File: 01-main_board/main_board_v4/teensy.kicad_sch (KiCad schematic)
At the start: 15 parts, among them IC8 AD8591ARTZ-REEL7, U1 Teensy4.1, U3 MCP2562FD-E/SN

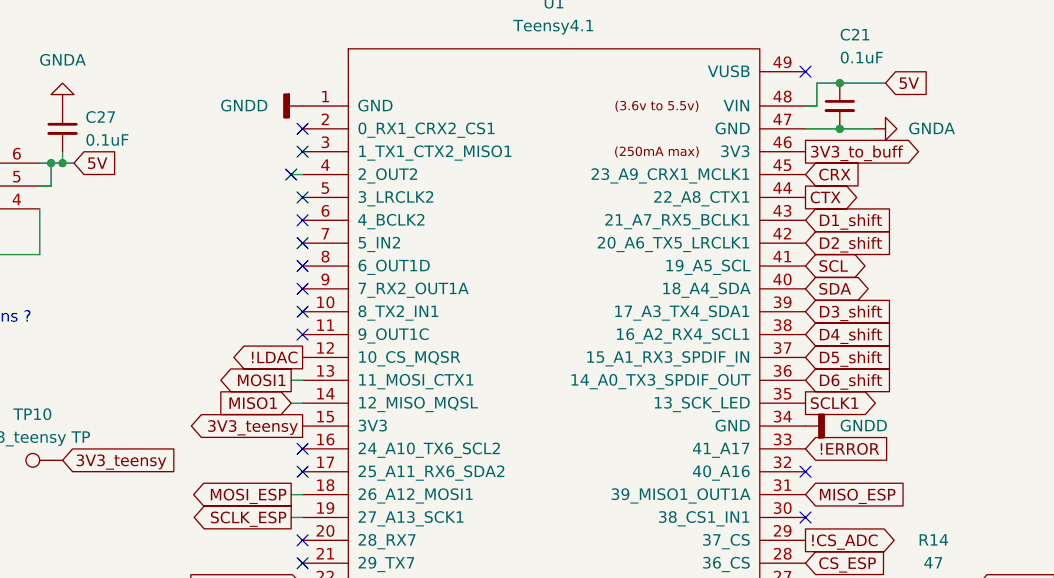
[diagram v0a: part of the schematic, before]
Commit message: regenerated gerbers
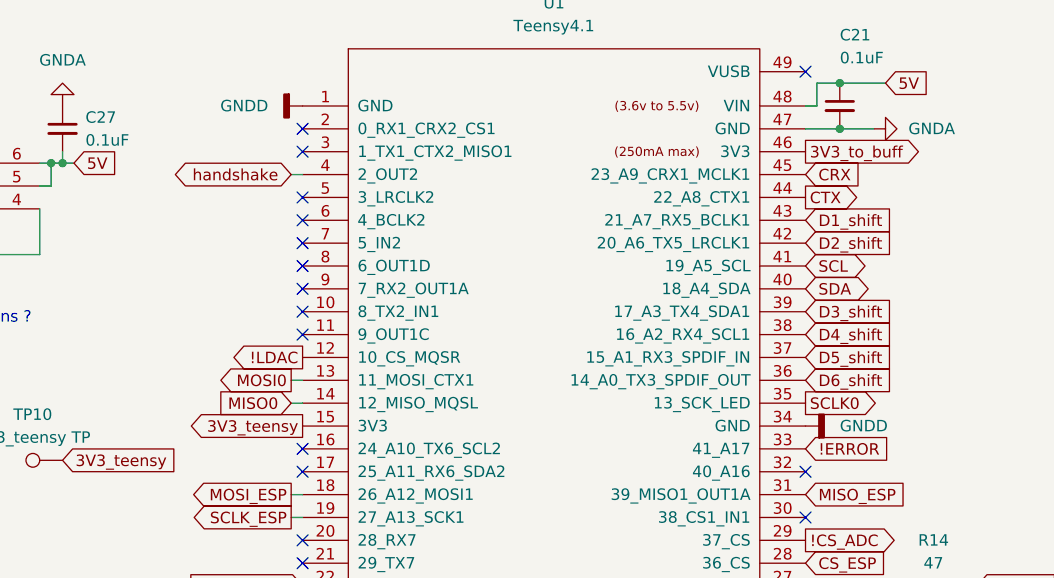
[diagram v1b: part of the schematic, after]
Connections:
- net handshake: now reaches U1.4 (2_OUT2)
- net MISO1 renamed MISO0
- net MOSI1 renamed MOSI0
- net SCLK1 renamed SCLK0
- no-connect marks 27 -> 26
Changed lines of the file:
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@@
-	)
-	(no_connect
-		(at 181.61 46.99)
 	)
 	(no_connect
@@
 		)
 	)
-	(global_label "MOSI1"
+	(global_label "MOSI0"
 		(shape output)
 		(at 181.61 69.85 180)
@@
 		)
 	)
-	(global_label "MISO1"
+	(global_label "MISO0"
 		(shape input)
 		(at 181.61 72.39 180)
@@
 		)
 	)
+	(global_label "handshake"
+		(shape bidirectional)
+		(at 181.61 46.99 180)
+		(fields_autoplaced yes)
+		(effects
+			(font
+				(size 1.27 1.27)
+			)
+			(justify right)
+		)
+		(property "Intersheetrefs" "${INTERSHEET_REFS}"
+			(at 167.4747 46.99 0)
+			(effects
+				(font
+					(size 1.27 1.27)
+				)
+				(justify right)
+				(hide yes)
+			)
+		)
+	)
 	(global_label "D2_shift"
 		(shape input)
@@
 		)
 	)
-	(global_label "SCLK1"
+	(global_label "SCLK0"
 		(shape output)
 		(at 238.76 72.39 0)
